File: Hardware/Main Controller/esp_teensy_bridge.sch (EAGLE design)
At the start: 55 parts, among them IC1 BQ79600PWRQ1, Q1 SI7611DN-T1-GE3, Q2 SI7611DN-T1-GE3, Q3 SI7611DN-T1-GE3

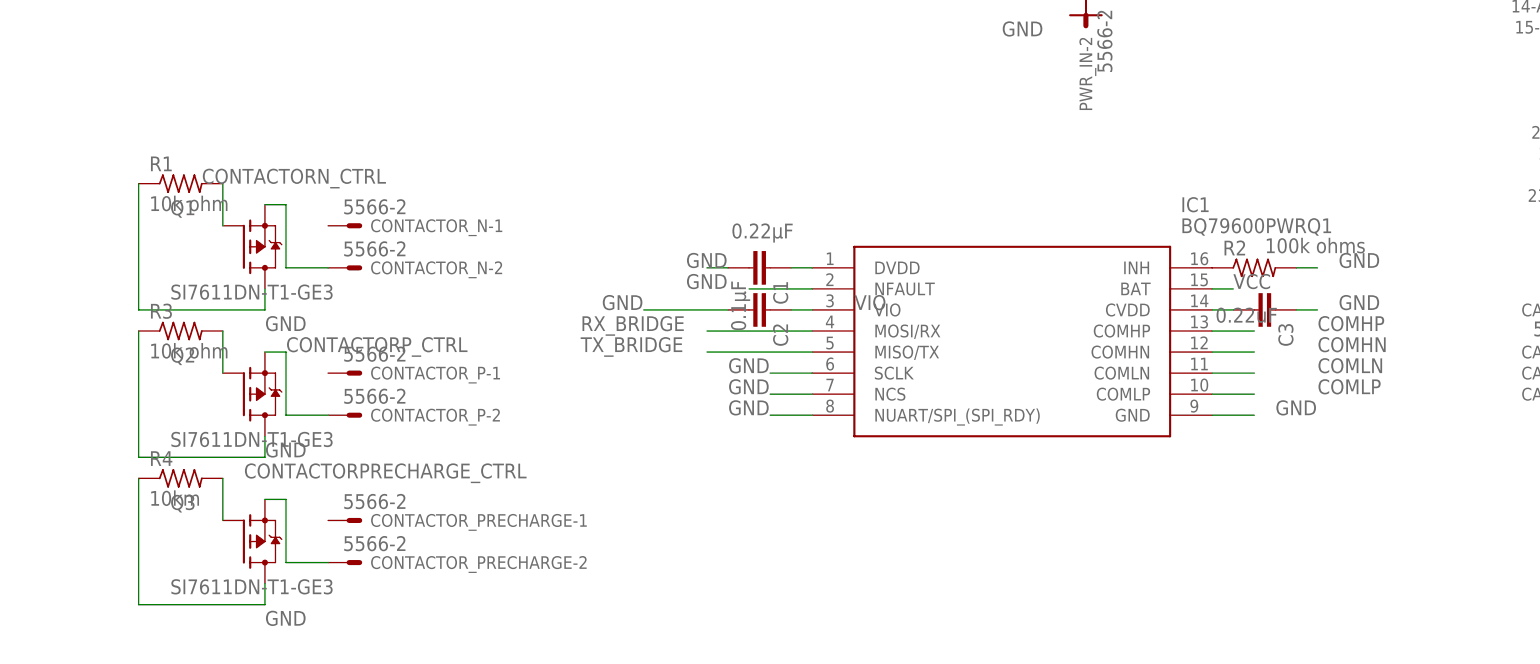
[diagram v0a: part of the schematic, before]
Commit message: layout changes to main
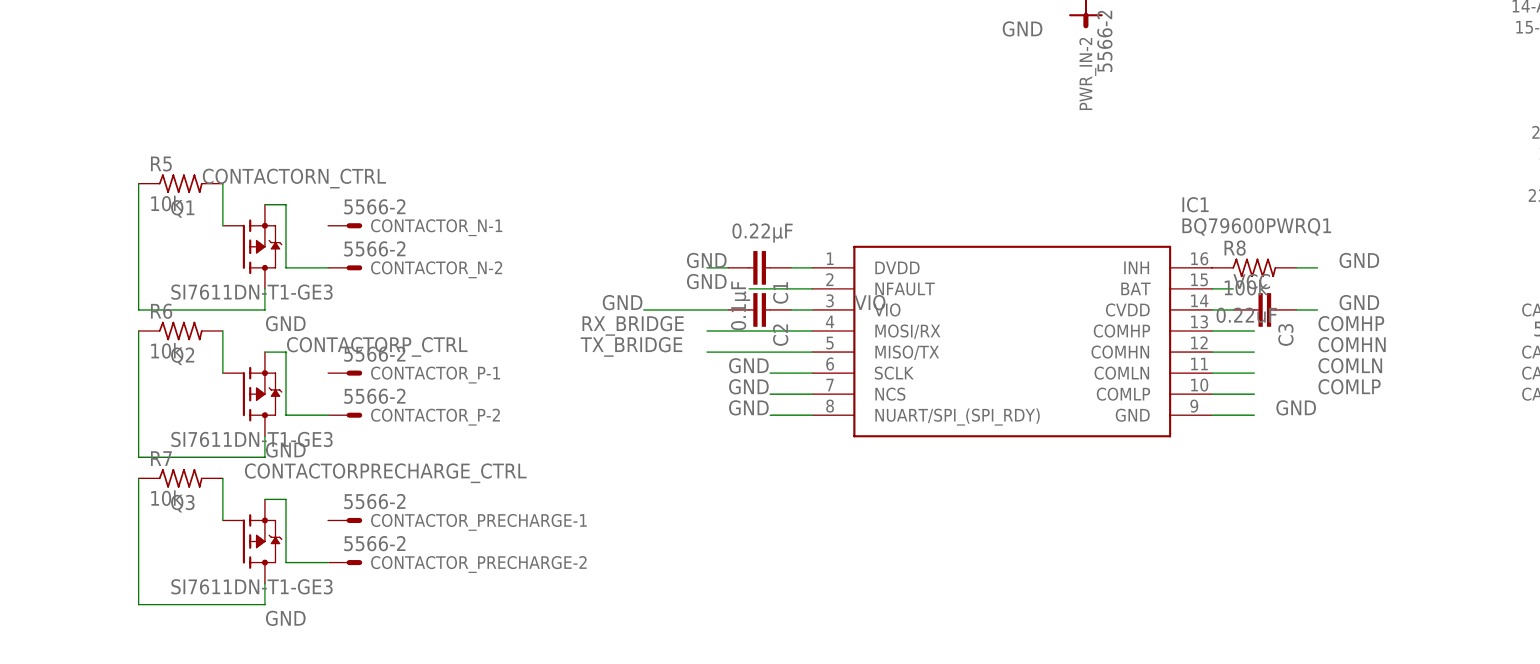
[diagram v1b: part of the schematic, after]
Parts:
- removed R1, R3: 10k ohm, rcl:R-US_0204/2V
- removed R2: 100k ohms, rcl:R-US_0204/7
- removed R4: 10km, rcl:R-US_0204/2V
- added R5, R6, R7: 10k, rcl:R-US_R0603
- added R8: 100k, rcl:R-US_R0603
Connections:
- net CONTACTORN_CTRL: now also R5.2; no longer R1.2
- net CONTACTORPRECHARGE_CTRL: now also R7.2; no longer R4.2
- net CONTACTORP_CTRL: now also R6.2; no longer R3.2
- net GND: now also R5.1, R6.1, R7.1, R8.2; no longer R1.1, R2.2, R3.1, R4.1
- net N$4: now also R8.1; no longer R2.1
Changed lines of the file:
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@@
 <part name="C2" library="capacitor-wima" library_urn="urn:adsk.eagle:library:116" deviceset="C" device="2,5-3" package3d_urn="urn:adsk.eagle:package:5436/1" value="0.1μF"/>
 <part name="C3" library="capacitor-wima" library_urn="urn:adsk.eagle:library:116" deviceset="C" device="2.5/2" package3d_urn="urn:adsk.eagle:package:5415/1" value="0.22uF"/>
-<part name="R2" library="rcl" library_urn="urn:adsk.eagle:library:334" deviceset="R-US_" device="0204/7" package3d_urn="urn:adsk.eagle:package:23498/2" value="100k ohms"/>
 <part name="TME1205S" library="dc-dc-converter" library_urn="urn:adsk.eagle:library:208" deviceset="NME" device="" package3d_urn="urn:adsk.eagle:package:12313/1"/>
 <part name="GND1" library="supply1" library_urn="urn:adsk.eagle:library:371" deviceset="GND" device=""/>
@@
 <part name="Q2" library="SI7611DN-T1-GE3" deviceset="SI7611DN-T1-GE3" device=""/>
 <part name="Q3" library="SI7611DN-T1-GE3" deviceset="SI7611DN-T1-GE3" device=""/>
-<part name="R1" library="rcl" library_urn="urn:adsk.eagle:library:334" deviceset="R-US_" device="0204/2V" package3d_urn="urn:adsk.eagle:package:23495/1" value="10k ohm"/>
-<part name="R3" library="rcl" library_urn="urn:adsk.eagle:library:334" deviceset="R-US_" device="0204/2V" package3d_urn="urn:adsk.eagle:package:23495/1" value="10k ohm"/>
-<part name="R4" library="rcl" library_urn="urn:adsk.eagle:library:334" deviceset="R-US_" device="0204/2V" package3d_urn="urn:adsk.eagle:package:23495/1" value="10km"/>
 <part name="RCOML" library="rcl" library_urn="urn:adsk.eagle:library:334" deviceset="R-US_" device="R0603" package3d_urn="urn:adsk.eagle:package:23555/3" value="1k"/>
 <part name="CCOMLNG" library="rcl" library_urn="urn:adsk.eagle:library:334" deviceset="C-EU" device="C0603" package3d_urn="urn:adsk.eagle:package:23616/2" value="220 pF"/>
@@
 <part name="ESDCOMH" library="ESDAVLC6-2BLY" deviceset="ESDAVLC6-2BLY" device=""/>
 <part name="COML2" library="con-molex" library_urn="urn:adsk.eagle:library:165" deviceset="5566-2" device="" package3d_urn="urn:adsk.eagle:package:8078583/1"/>
+<part name="R5" library="rcl" library_urn="urn:adsk.eagle:library:334" deviceset="R-US_" device="R0603" package3d_urn="urn:adsk.eagle:package:23555/3" value="10k"/>
+<part name="R6" library="rcl" library_urn="urn:adsk.eagle:library:334" deviceset="R-US_" device="R0603" package3d_urn="urn:adsk.eagle:package:23555/3" value="10k"/>
+<part name="R7" library="rcl" library_urn="urn:adsk.eagle:library:334" deviceset="R-US_" device="R0603" package3d_urn="urn:adsk.eagle:package:23555/3" value="10k"/>
+<part name="R8" library="rcl" library_urn="urn:adsk.eagle:library:334" deviceset="R-US_" device="R0603" package3d_urn="urn:adsk.eagle:package:23555/3" value="100k"/>
 </parts>
 <sheets>
@@
 <attribute name="VALUE" x="-14.859" y="59.436" size="1.778" layer="96"/>
 </instance>
-<instance part="R2" gate="G$1" x="-10.16" y="66.04" smashed="yes">
-<attribute name="NAME" x="-13.97" y="67.5386" size="1.778" layer="95"/>
-<attribute name="VALUE" x="-8.89" y="67.818" size="1.778" layer="96"/>
-</instance>
 <instance part="TME1205S" gate="G$1" x="-30.48" y="111.76" smashed="yes">
 <attribute name="NAME" x="-40.64" y="117.475" size="1.778" layer="95"/>
@@
 <attribute name="NAME" x="-140.987490625" y="36.837490625" size="1.7815" layer="95"/>
 </instance>
-<instance part="R1" gate="G$1" x="-139.7" y="76.2" smashed="yes">
-<attribute name="NAME" x="-143.51" y="77.6986" size="1.778" layer="95"/>
-<attribute name="VALUE" x="-143.51" y="72.898" size="1.778" layer="96"/>
-</instance>
-<instance part="R3" gate="G$1" x="-139.7" y="58.42" smashed="yes">
-<attribute name="NAME" x="-143.51" y="59.9186" size="1.778" layer="95"/>
-<attribute name="VALUE" x="-143.51" y="55.118" size="1.778" layer="96"/>
-</instance>
-<instance part="R4" gate="G$1" x="-139.7" y="40.64" smashed="yes">
-<attribute name="NAME" x="-143.51" y="42.1386" size="1.778" layer="95"/>
-<attribute name="VALUE" x="-143.51" y="37.338" size="1.778" layer="96"/>
-</instance>
 <instance part="RCOML" gate="G$1" x="-200.66" y="-22.86" smashed="yes" rot="R180">
 <attribute name="NAME" x="-196.85" y="-24.3586" size="1.778" layer="95" rot="R180"/>
@@
 <attribute name="NAME" x="-173.482" y="-68.58" size="1.524" layer="95" rot="R270"/>
 <attribute name="VALUE" x="-171.323" y="-65.278" size="1.778" layer="96" rot="R270"/>
+</instance>
+<instance part="R5" gate="G$1" x="-139.7" y="76.2" smashed="yes">
+<attribute name="NAME" x="-143.51" y="77.6986" size="1.778" layer="95"/>
+<attribute name="VALUE" x="-143.51" y="72.898" size="1.778" layer="96"/>
+</instance>
+<instance part="R6" gate="G$1" x="-139.7" y="58.42" smashed="yes">
+<attribute name="NAME" x="-143.51" y="59.9186" size="1.778" layer="95"/>
+<attribute name="VALUE" x="-143.51" y="55.118" size="1.778" layer="96"/>
+</instance>
+<instance part="R7" gate="G$1" x="-139.7" y="40.64" smashed="yes">
+<attribute name="NAME" x="-143.51" y="42.1386" size="1.778" layer="95"/>
+<attribute name="VALUE" x="-143.51" y="37.338" size="1.778" layer="96"/>
+</instance>
+<instance part="R8" gate="G$1" x="-10.16" y="66.04" smashed="yes">
+<attribute name="NAME" x="-13.97" y="67.5386" size="1.778" layer="95"/>
+<attribute name="VALUE" x="-13.97" y="62.738" size="1.778" layer="96"/>
 </instance>
 </instances>
@@
 </segment>
 <segment>
-<pinref part="R2" gate="G$1" pin="2"/>
 <wire x1="-5.08" y1="66.04" x2="-2.54" y2="66.04" width="0.1524" layer="91"/>
 <label x="0" y="66.04" size="1.778" layer="95"/>
+<pinref part="R8" gate="G$1" pin="2"/>
 </segment>
 <segment>
@@
 <label x="-129.54" y="58.42" size="1.778" layer="95"/>
 <wire x1="-129.54" y1="60.96" x2="-144.78" y2="60.96" width="0.1524" layer="91"/>
-<pinref part="R1" gate="G$1" pin="1"/>
 <wire x1="-144.78" y1="76.2" x2="-144.78" y2="60.96" width="0.1524" layer="91"/>
+<pinref part="R5" gate="G$1" pin="1"/>
 </segment>
 <segment>
@@
 <wire x1="-129.54" y1="45.72" x2="-129.54" y2="43.18" width="0.1524" layer="91"/>
 <label x="-129.54" y="43.18" size="1.778" layer="95"/>
-<pinref part="R3" gate="G$1" pin="1"/>
 <wire x1="-144.78" y1="58.42" x2="-144.78" y2="43.18" width="0.1524" layer="91"/>
 <wire x1="-144.78" y1="43.18" x2="-129.54" y2="43.18" width="0.1524" layer="91"/>
+<pinref part="R6" gate="G$1" pin="1"/>
 </segment>
 <segment>
@@
 <wire x1="-129.54" y1="27.94" x2="-129.54" y2="25.4" width="0.1524" layer="91"/>
 <label x="-129.54" y="22.86" size="1.778" layer="95"/>
-<pinref part="R4" gate="G$1" pin="1"/>
 <wire x1="-144.78" y1="40.64" x2="-144.78" y2="25.4" width="0.1524" layer="91"/>
 <wire x1="-144.78" y1="25.4" x2="-129.54" y2="25.4" width="0.1524" layer="91"/>
+<pinref part="R7" gate="G$1" pin="1"/>
 </segment>
 <segment>
@@
 <pinref part="C3" gate="G$1" pin="2"/>
 <wire x1="-15.24" y1="60.96" x2="-12.7" y2="60.96" width="0.1524" layer="91"/>
-</segment>
-</net>
-<net name="N$4" class="0">
-<segment>
-<pinref part="IC1" gate="G$1" pin="INH"/>
-<pinref part="R2" gate="G$1" pin="1"/>
 </segment>
 </net>
@@
 <wire x1="-134.62" y1="71.12" x2="-134.62" y2="76.2" width="0.1524" layer="91"/>
 <label x="-137.16" y="76.2" size="1.778" layer="95"/>
-<pinref part="R1" gate="G$1" pin="2"/>
+<pinref part="R5" gate="G$1" pin="2"/>
 </segment>
 <segment>
@@
 <pinref part="Q2" gate="G$1" pin="G"/>
 <wire x1="-134.62" y1="53.34" x2="-134.62" y2="58.42" width="0.1524" layer="91"/>
-<pinref part="R3" gate="G$1" pin="2"/>
 <label x="-127" y="55.88" size="1.778" layer="95"/>
+<pinref part="R6" gate="G$1" pin="2"/>
 </segment>
 <segment>
@@
 <net name="CONTACTORPRECHARGE_CTRL" class="0">
 <segment>
-<pinref part="R4" gate="G$1" pin="2"/>
 <pinref part="Q3" gate="G$1" pin="G"/>
 <wire x1="-134.62" y1="40.64" x2="-134.62" y2="35.56" width="0.1524" layer="91"/>
 <label x="-132.08" y="40.64" size="1.778" layer="95"/>
+<pinref part="R7" gate="G$1" pin="2"/>
 </segment>
 <segment>
@@
 </segment>
 </net>
+<net name="N$4" class="0">
+<segment>
+<pinref part="IC1" gate="G$1" pin="INH"/>
+<pinref part="R8" gate="G$1" pin="1"/>
+</segment>
+</net>
